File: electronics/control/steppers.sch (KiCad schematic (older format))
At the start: 53 parts, among them Q1 SH8K5, Q2 SH8K5, Q3 SH8K5, Q4 SH8K5, Q5 SH8K5, U2 MOCD217R2M, U3 MOCD217R2M, U4 MOCD217R2M, U5 MOCD217R2M, U6 MOCD217R2M

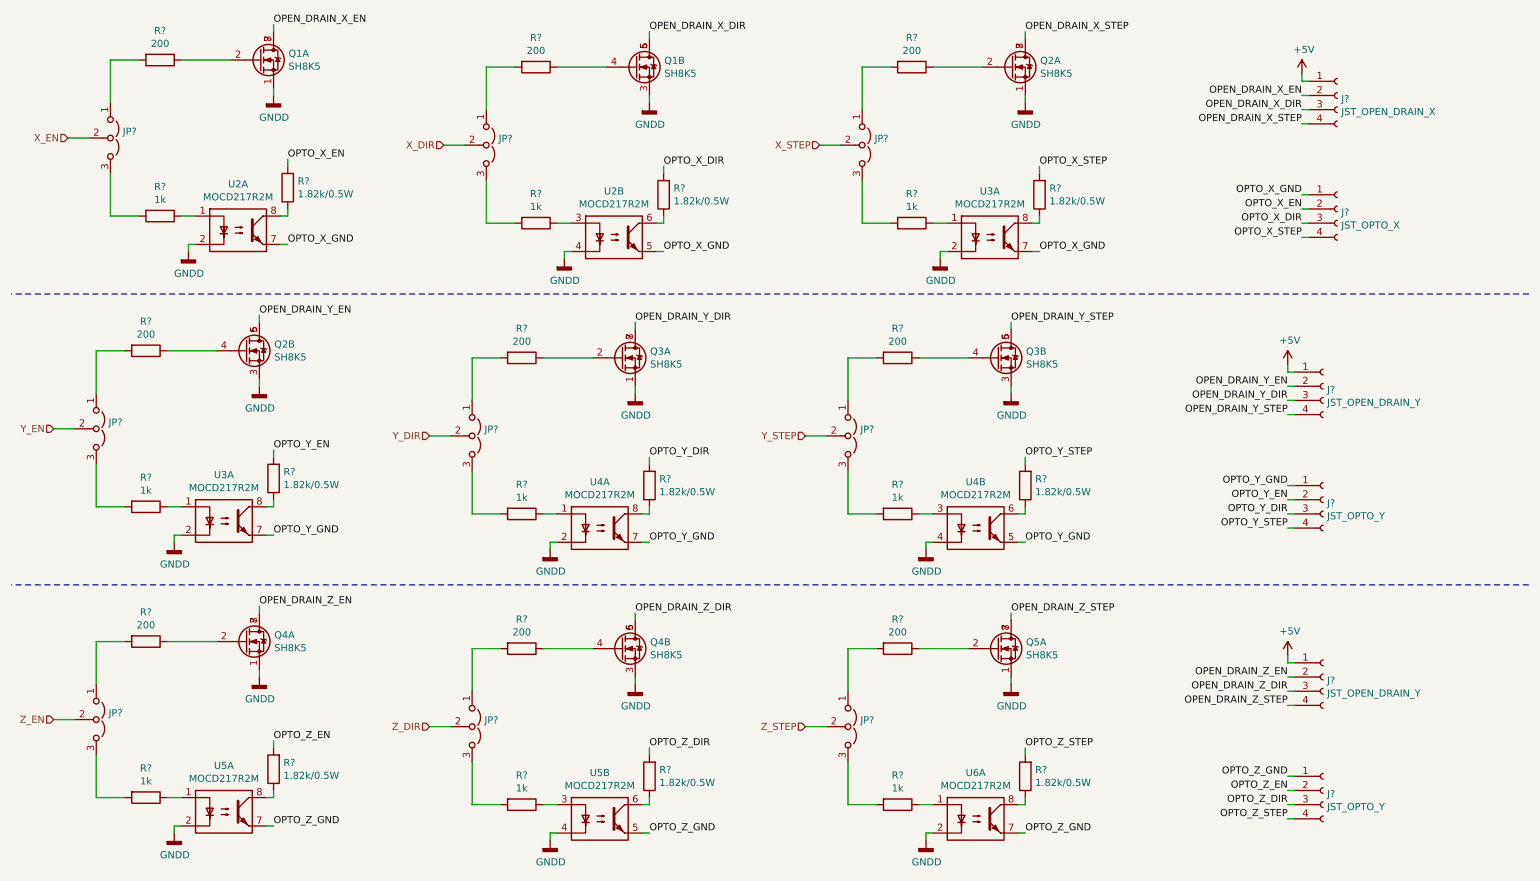
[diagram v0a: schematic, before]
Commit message: Add the PCB.
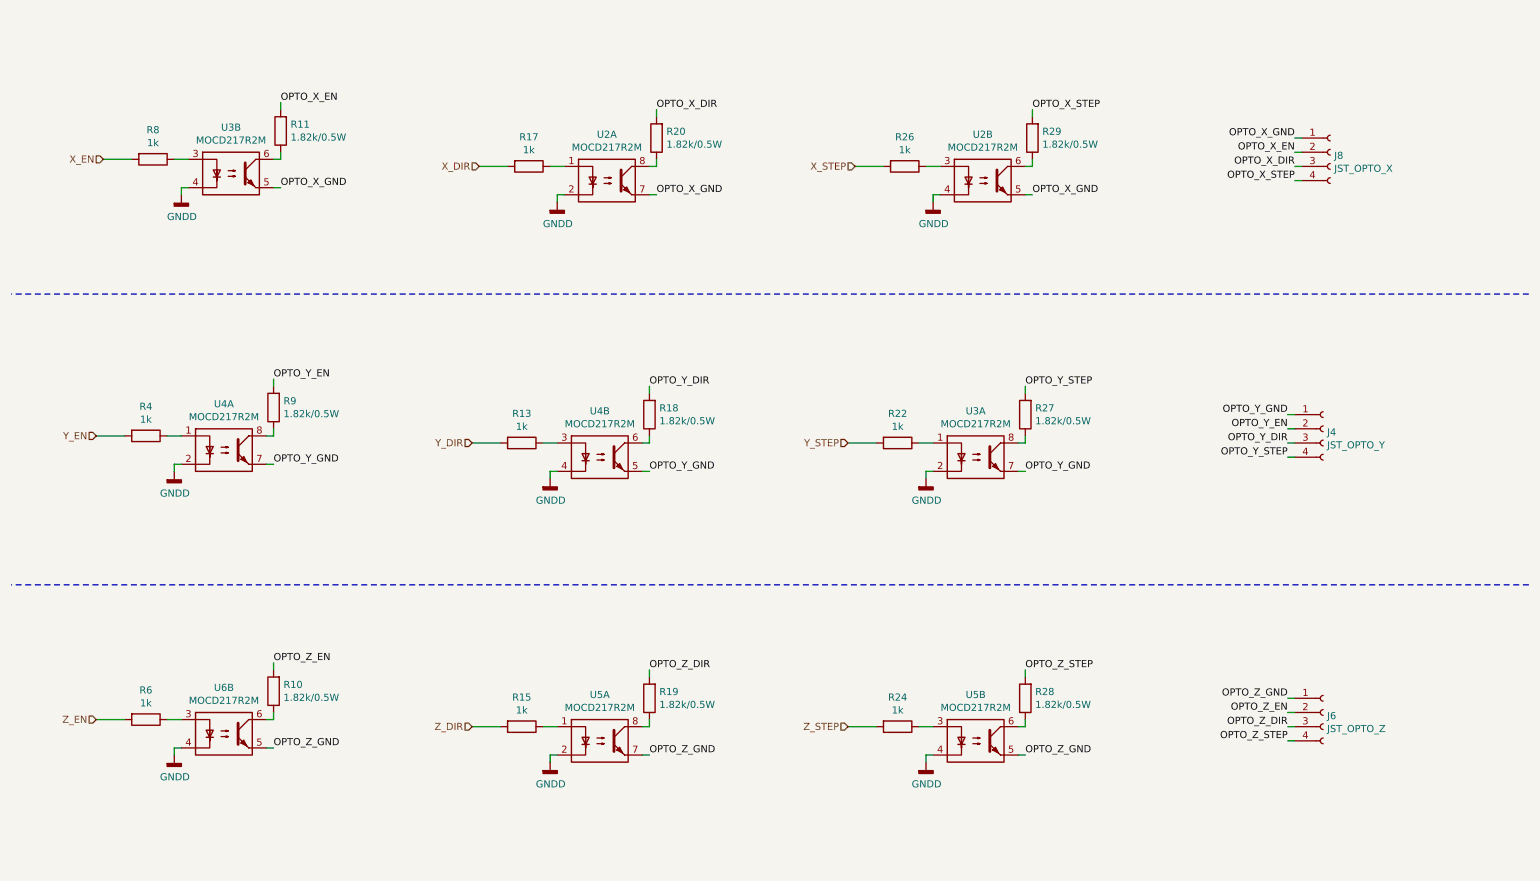
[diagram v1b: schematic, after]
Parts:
- removed J?: JST_OPEN_DRAIN_X, symbol Connector:Conn_01x04_Female
- removed J? (x2): JST_OPEN_DRAIN_Y, symbol Connector:Conn_01x04_Female
- removed JP? (x9): Jumper_3_Open, symbol Jumper:Jumper_3_Open
- removed Q1, Q2, Q3, Q4, Q5: SH8K5, symbol CNC:SH8K5
- removed R? (x9): 200, symbol Device:R
- J4, J8: renamed from J?; footprint (none) -> Connector_JST:JST_XH_B4B-XH-A_1x04_P2.50mm_Vertical
- J6: renamed from J?; value JST_OPTO_Y -> JST_OPTO_Z; footprint (none) -> Connector_JST:JST_XH_B4B-XH-A_1x04_P2.50mm_Vertical
- R10, R11, R18, R19, R20, R27, R28, R29, R9: renamed from R?; footprint (none) -> Resistor_SMD:R_1210_3225Metric
- R13, R15, R17, R22, R24, R26, R4, R6, R8: renamed from R?; footprint (none) -> Resistor_SMD:R_0805_2012Metric
- U2, U4, U5: footprint (none) -> Package_SO:SOIC-8_3.9x4.9mm_P1.27mm
- U2, U4: renamed from U3; footprint (none) -> Package_SO:SOIC-8_3.9x4.9mm_P1.27mm
- U3: renamed from U2; footprint (none) -> Package_SO:SOIC-8_3.9x4.9mm_P1.27mm
- U3: renamed from U4; footprint (none) -> Package_SO:SOIC-8_3.9x4.9mm_P1.27mm
- U5: renamed from U6; footprint (none) -> Package_SO:SOIC-8_3.9x4.9mm_P1.27mm
- U6: renamed from U5; footprint (none) -> Package_SO:SOIC-8_3.9x4.9mm_P1.27mm
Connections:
- net GNDD: now also U2.2, U2.4, U3.2, U3.4, U4.4, U5.2, U5.4, U6.4; no longer U2.2, U2.4, U3.2, U3.4, U4.2, U5.2, U5.4, U6.2
- net OPTO_X_GND: now also U2.5, U2.7, U3.5; no longer U2.5, U2.7, U3.7
- net OPTO_Y_GND: now also U3.7, U4.5; no longer U3.5, U4.7
- net OPTO_Z_GND: now also U5.5, U5.7, U6.5; no longer U5.5, U5.7, U6.7
- net X_DIR: now also R17.2
- net X_EN: now also R8.2
- net X_STEP: now also R26.2
- net Y_DIR: now also R13.2
- net Y_EN: now also R4.2
- net Y_STEP: now also R22.2
- net Z_DIR: now also R15.2
- net Z_EN: now also R6.2
- net Z_STEP: now also R24.2
- net at R17.1: now also U2.1; no longer U2.3
- net at R20.1: now also U2.8; no longer U2.6
- net at R26.1: now also U2.3; no longer U2.1
- net at R29.1: now also U2.6; no longer U2.8
- net at R8.1: now also U3.3; no longer U3.1
- net at R11.1: now also U3.6; no longer U3.8
- net at R13.1: now also U4.3; no longer U4.1
- net at R18.1: now also U4.6; no longer U4.8
- net at R22.1: now also U3.1; no longer U3.3
- net at R27.1: now also U3.8; no longer U3.6
- net at R6.1: now also U6.3; no longer U6.1
- net at R10.1: now also U6.6; no longer U6.8
- net at R15.1: now also U5.1; no longer U5.3
- net at R19.1: now also U5.8; no longer U5.6
- net at R24.1: now also U5.3; no longer U5.1
- net at R28.1: now also U5.6; no longer U5.8
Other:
- moved on the sheet: J4, J6, J8, R10, R11, R13, R15, R17, R18, R19, R20, R22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
